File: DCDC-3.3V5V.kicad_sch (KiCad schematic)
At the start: 22 parts, among them J1 Conn_01x02, J2 Conn_01x02, U1 TPS63020DSJR, U2 TPS63020DSJR

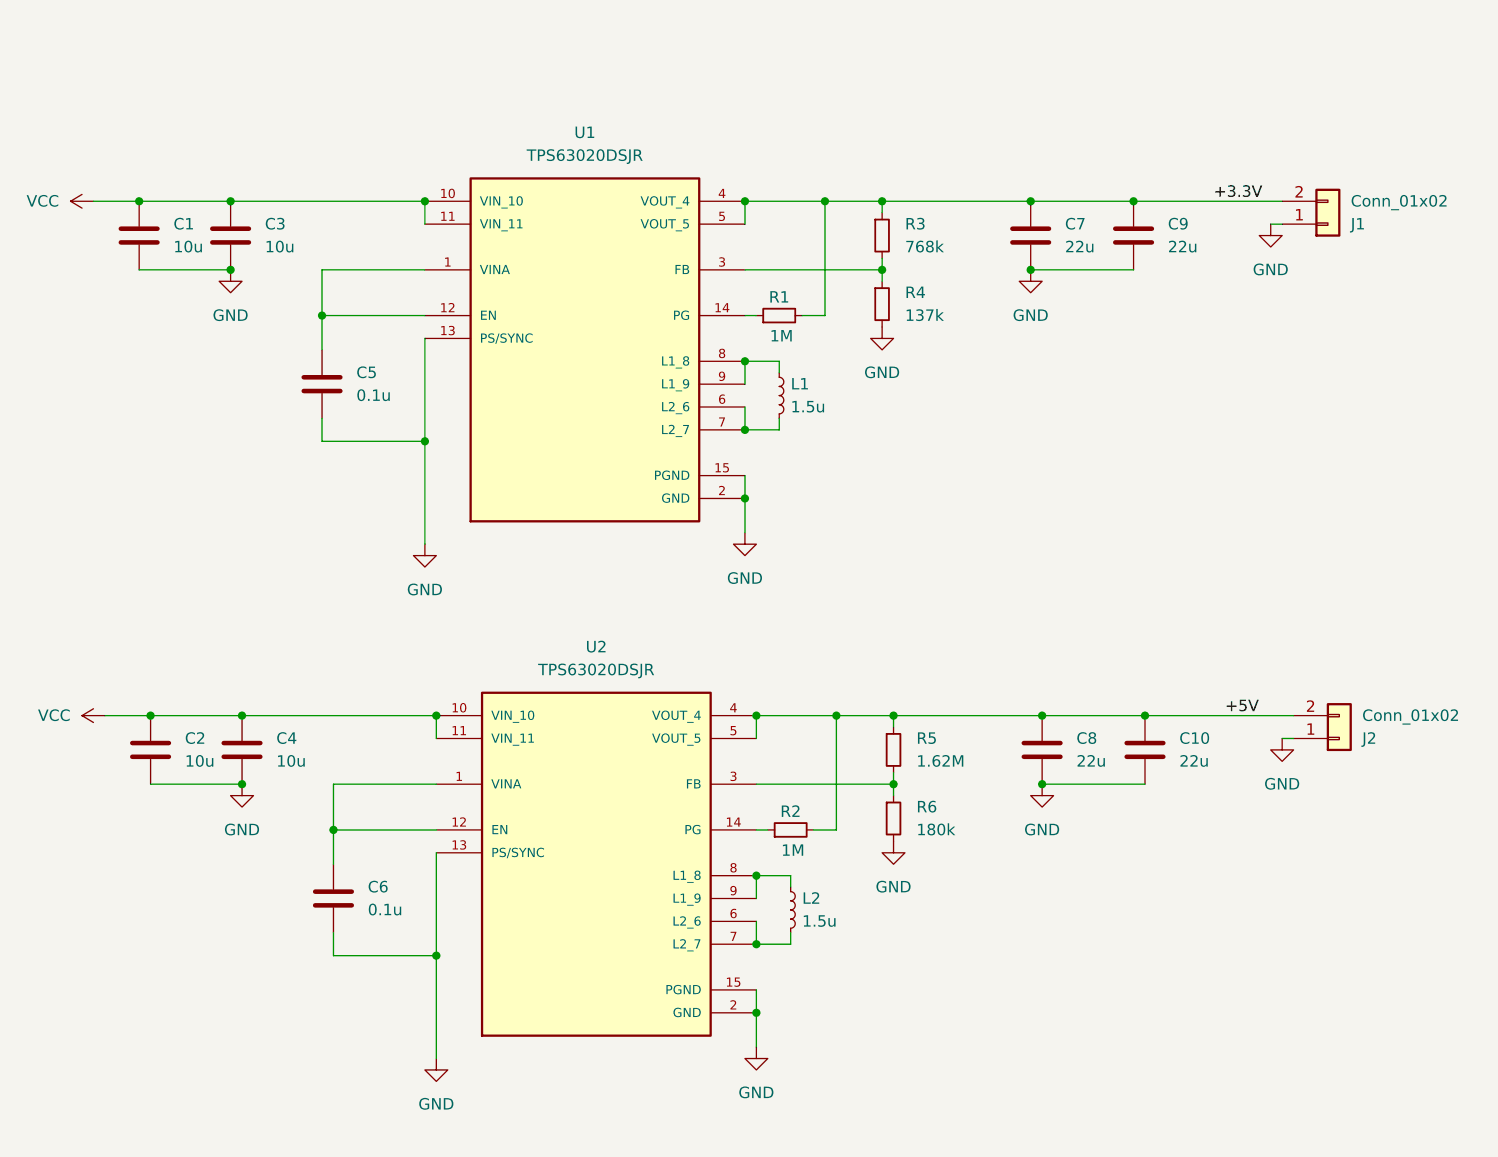
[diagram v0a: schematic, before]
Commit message: update
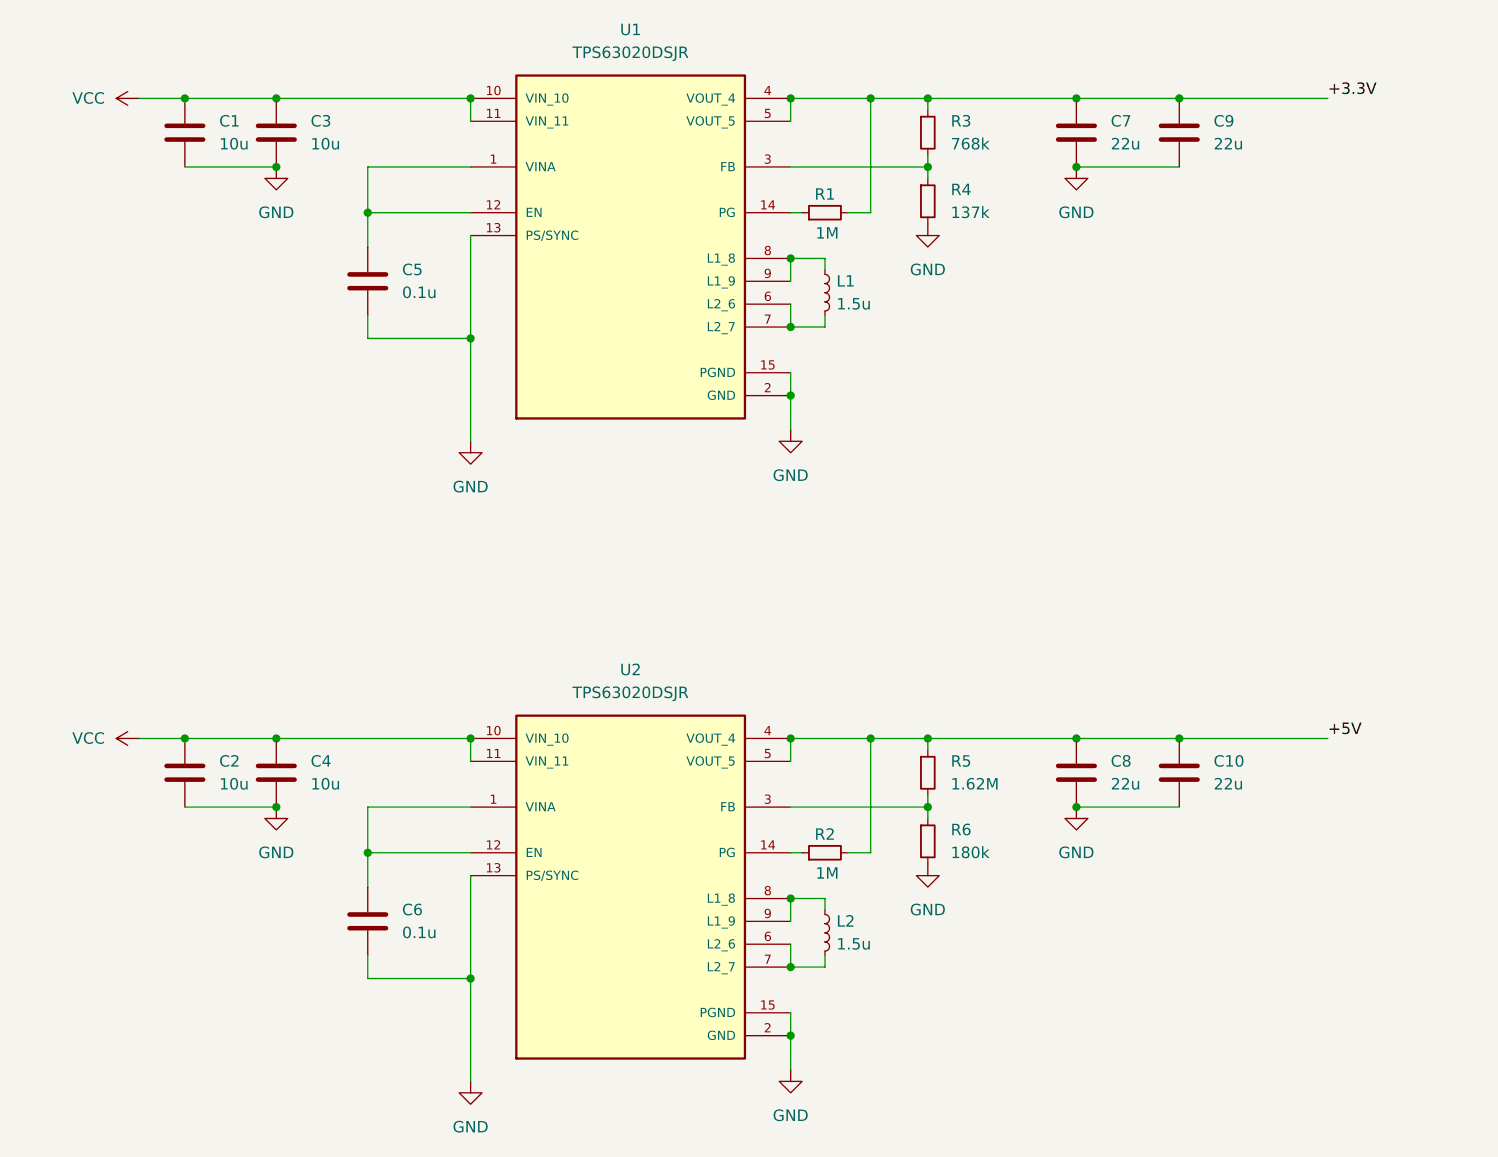
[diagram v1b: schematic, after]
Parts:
- removed J1, J2: Conn_01x02, Connector_JST:JST_XA_B02B-XASK-1_1x02_P2.50mm_Vertical, symbol Connector_Generic:Conn_01x02
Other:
- moved on the sheet: C1, C10, C2, C3, C4, C5, C6, C7, C8, C9, L1, L2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
